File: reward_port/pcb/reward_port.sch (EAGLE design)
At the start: 16 parts, among them U2 ATTINY2313A

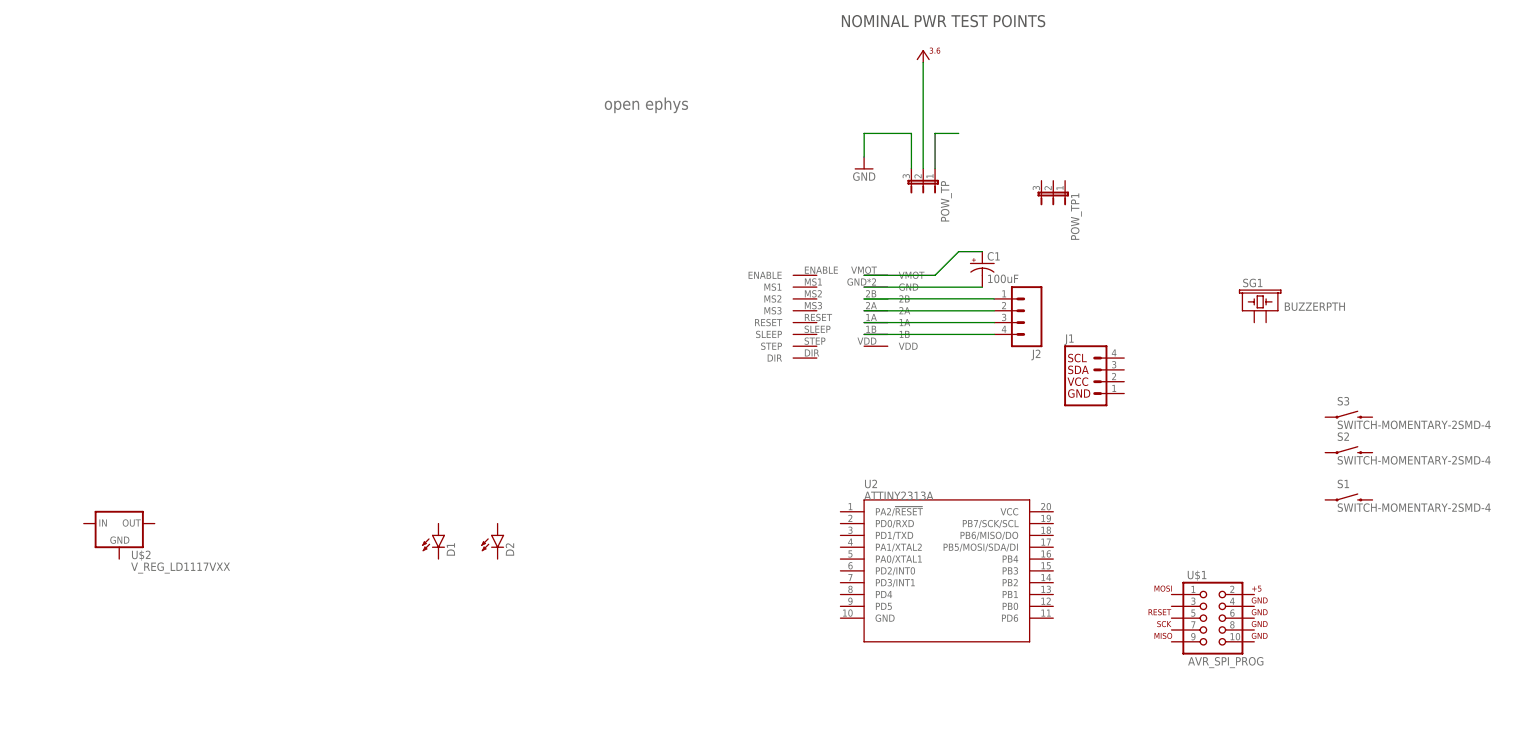
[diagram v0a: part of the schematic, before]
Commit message: more schematic layout
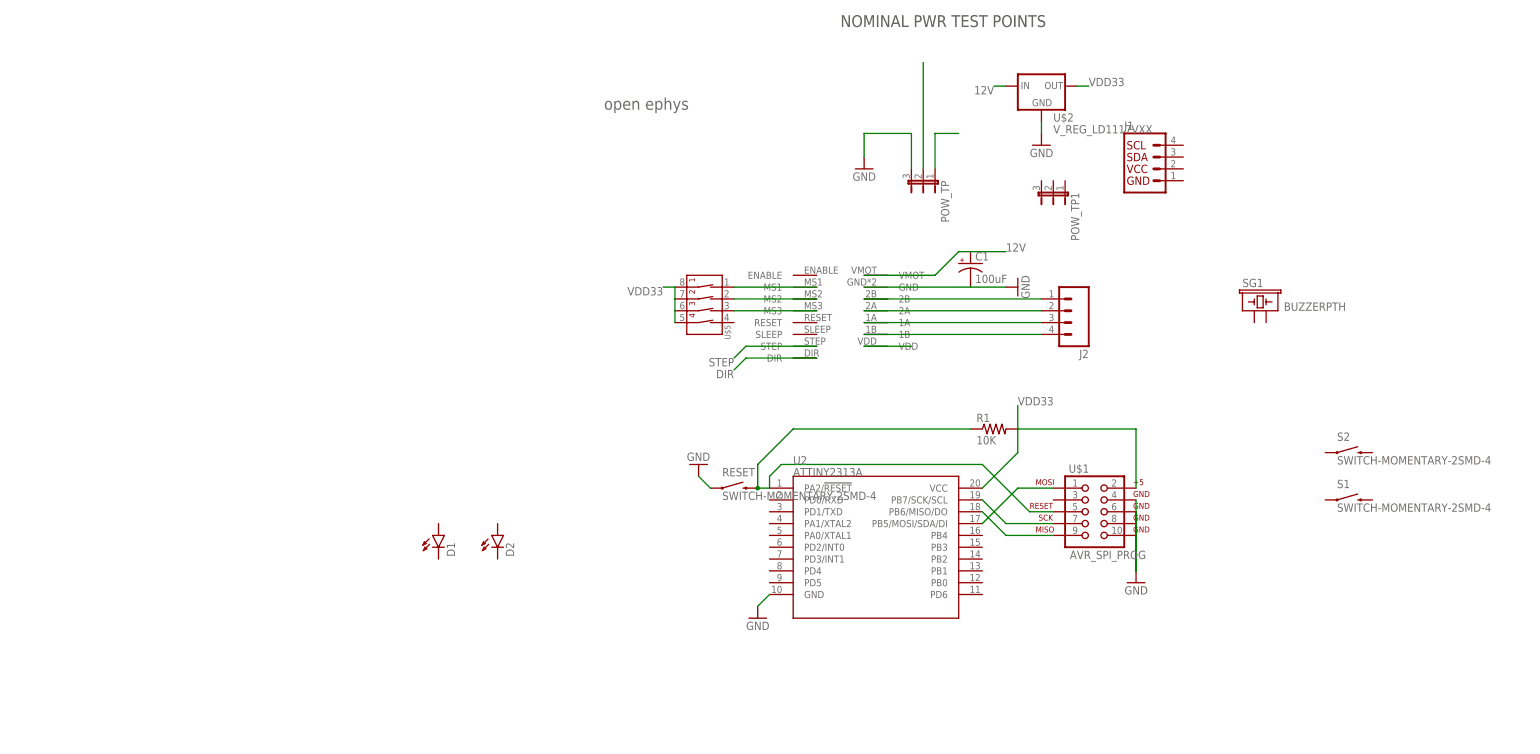
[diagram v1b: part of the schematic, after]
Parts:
- removed S3: SWITCH-MOMENTARY-2SMD-4, SparkFun-Electromechanical:SWITCH-MOMENTARY-2SMD-4
- added R1: 10K, SparkFun-Resistors:10KOHM-1/10W-1%(0603)0603
- added RESET: SWITCH-MOMENTARY-2SMD-4, SparkFun-Electromechanical:SWITCH-MOMENTARY-2SMD-4
- added U$5: 4-POS-DIP, SparkFun-Electromechanical:4-POS-DIP
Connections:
- net +3V6 renamed N$10
- removed net N$5: C1.-, U$3.GND
- new net 12V: C1.+, U$2.IN, U$3.VMOT
- new net DIR: U$3.DIR
- new net N$11: U$3.MS1, U$5.1A
- new net N$12: U$3.MS2, U$5.2A
- new net N$13: U$3.MS3, U$5.3A
- new net N$14: U$1.7, U2.PB7/SCK/SCL
- new net N$15: U$1.9, U2.PB6/MISO/DO
- new net N$16: U$1.1, U2.PB5/MOSI/SDA/DI
- new net STEP: U$3.STEP
- new net VDD33: R1.2, U$1.2, U$2.OUT, U$3.VDD, U$5.1B, U$5.2B, U$5.3B, U$5.4B, U2.VCC
- net GND: now also C1.-, RESET.1, U$1.10, U$1.4, U$1.6, U$1.8, U$2.GND, U$3.GND, U2.GND
- net N$4: now also R1.1, RESET.2, U$1.5, U2.PA2/!RESET; no longer C1.+, U$3.VMOT
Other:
- moved on the sheet: C1, J1, J2, U$1, U$2, U2
